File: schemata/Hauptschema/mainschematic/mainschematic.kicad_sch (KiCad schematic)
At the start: 11 parts, among them M1 Stepper_Motor_bipolar, M2 Stepper_Motor_bipolar, M3 Lager ROT, M4 Lager GRÜN, M5 Lager BLAU, M6 Zentrierschieber 1, M7 Zentrierschieber 2

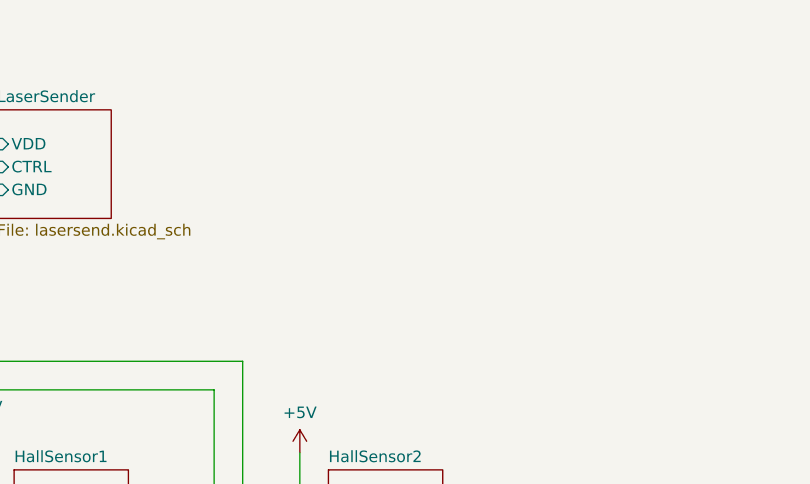
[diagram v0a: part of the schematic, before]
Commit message: fixed main schematic :)
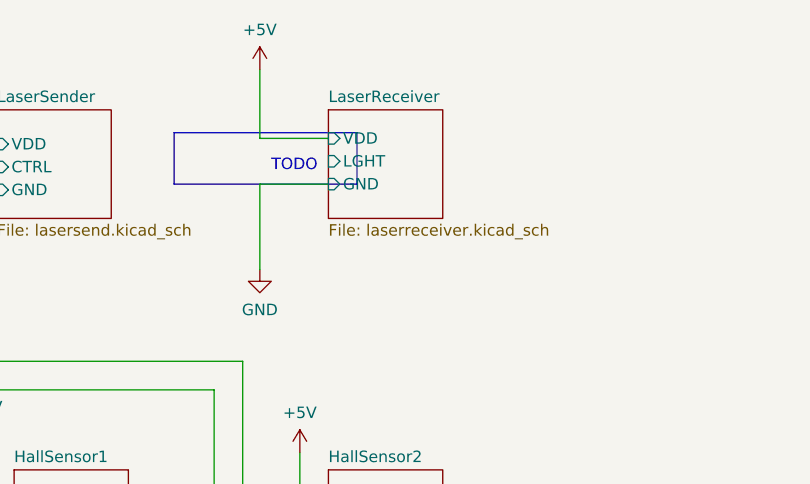
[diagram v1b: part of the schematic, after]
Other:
- added sheet LaserReceiver (laserreceiver.kicad_sch)
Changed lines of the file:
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@@
+    (stroke (width 0) (type default))
+  )
+  (wire (pts (xy 331.47 54.61) (xy 323.85 54.61))
     (stroke (width 0) (type default))
   )
@@
     (stroke (width 0) (type default))
   )
+  (wire (pts (xy 323.85 69.215) (xy 323.85 59.69))
+    (stroke (width 0) (type default))
+  )
   (wire (pts (xy 262.89 144.145) (xy 257.175 144.145))
     (stroke (width 0) (type default))
@@
     (stroke (width 0) (type default))
   )
+  (wire (pts (xy 323.85 59.69) (xy 331.47 59.69))
+    (stroke (width 0) (type default))
+  )
   (wire (pts (xy 181.61 85.09) (xy 191.77 85.09))
     (stroke (width 0) (type default))
@@
   )
   (wire (pts (xy 64.135 179.705) (xy 73.025 179.705))
+    (stroke (width 0) (type default))
+  )
+  (wire (pts (xy 323.85 54.61) (xy 323.85 46.99))
     (stroke (width 0) (type default))
   )
@@
     (fill (type none))
   )
+  (rectangle (start 314.325 53.975) (end 334.645 59.69)
+    (stroke (width 0) (type default) (color 255 0 0 1))
+    (fill (type none))
+  )
   (rectangle (start 233.68 161.925) (end 275.59 190.5)
     (stroke (width 0) (type default))
@@
   (text "Raspberry Display and Power\nIn-/Output" (at 234.315 166.37 0)
     (effects (font (size 1.27 1.27)) (justify left bottom))
+  )
+  (text "TODO" (at 325.12 58.42 0)
+    (effects (font (size 1.27 1.27) (color 255 0 0 1)) (justify left bottom))
   )
   (symbol (lib_id "Motor:Motor_Servo") (at 56.515 179.705 0) (mirror y) (unit 1)
@@
     )
   )
+  (symbol (lib_id "power:GND") (at 323.85 69.215 0) (unit 1)
+    (in_bom yes) (on_board yes) (dnp no) (fields_autoplaced)
+    (property "Reference" "#PWR058" (at 323.85 75.565 0)
+      (effects (font (size 1.27 1.27)) hide)
+    )
+    (property "Value" "GND" (at 323.85 73.66 0)
+      (effects (font (size 1.27 1.27)))
+    )
+    (property "Footprint" "" (at 323.85 69.215 0)
+      (effects (font (size 1.27 1.27)) hide)
+    )
+    (property "Datasheet" "" (at 323.85 69.215 0)
+      (effects (font (size 1.27 1.27)) hide)
+    )
+    (pin "1")
+    (instances
+      (project "mainschematic"
+        (path "/086318dd-19eb-4c26-88b2-e7f1a0e5d55a"
+          (reference "#PWR058") (unit 1)
+        )
+      )
+    )
+  )
   (symbol (lib_id "power:+5V") (at 287.02 47.625 0) (unit 1)
     (in_bom yes) (on_board yes) (dnp no) (fields_autoplaced)
@@
         (path "/086318dd-19eb-4c26-88b2-e7f1a0e5d55a"
           (reference "#PWR034") (unit 1)
+        )
+      )
+    )
+  )
+  (symbol (lib_id "power:+5V") (at 323.85 46.99 0) (unit 1)
+    (in_bom yes) (on_board yes) (dnp no) (fields_autoplaced)
+    (property "Reference" "#PWR057" (at 323.85 50.8 0)
+      (effects (font (size 1.27 1.27)) hide)
+    )
+    (property "Value" "+5V" (at 323.85 42.545 0)
+      (effects (font (size 1.27 1.27)))
+    )
+    (property "Footprint" "" (at 323.85 46.99 0)
+      (effects (font (size 1.27 1.27)) hide)
+    )
+    (property "Datasheet" "" (at 323.85 46.99 0)
+      (effects (font (size 1.27 1.27)) hide)
+    )
+    (pin "1")
+    (instances
+      (project "mainschematic"
+        (path "/086318dd-19eb-4c26-88b2-e7f1a0e5d55a"
+          (reference "#PWR057") (unit 1)
         )
       )
@@
       )
     )
+  )
+  (sheet (at 331.47 51.435) (size 12.7 12.065) (fields_autoplaced)
+    (stroke (width 0.1524) (type solid) (color 72 0 0 1))
+    (fill (color 255 255 194 1.0000))
+    (property "Sheetname" "LaserReceiver" (at 331.47 50.7234 0)
+      (effects (font (size 1.27 1.27)) (justify left bottom))
+    )
+    (property "Sheetfile" "laserreceiver.kicad_sch" (at 331.47 64.0846 0)
+      (effects (font (size 1.27 1.27)) (justify left top))
+    )
+    (pin "LGHT" input (at 331.47 57.15 180)
+      (effects (font (size 1.27 1.27)) (justify left))
+    )
+    (pin "VDD" input (at 331.47 54.61 180)
+      (effects (font (size 1.27 1.27)) (justify left))
+    )
+    (pin "GND" input (at 331.47 59.69 180)
+      (effects (font (size 1.27 1.27)) (justify left))
+    )
+    (instances
+      (project "mainschematic"
+        (path "/086318dd-19eb-4c26-88b2-e7f1a0e5d55a" (page "6"))
+      )
+    )
